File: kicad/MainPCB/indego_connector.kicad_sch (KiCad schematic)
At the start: 20 parts, among them U1 26SHC-B-1A, U2 24SHC-B-1A

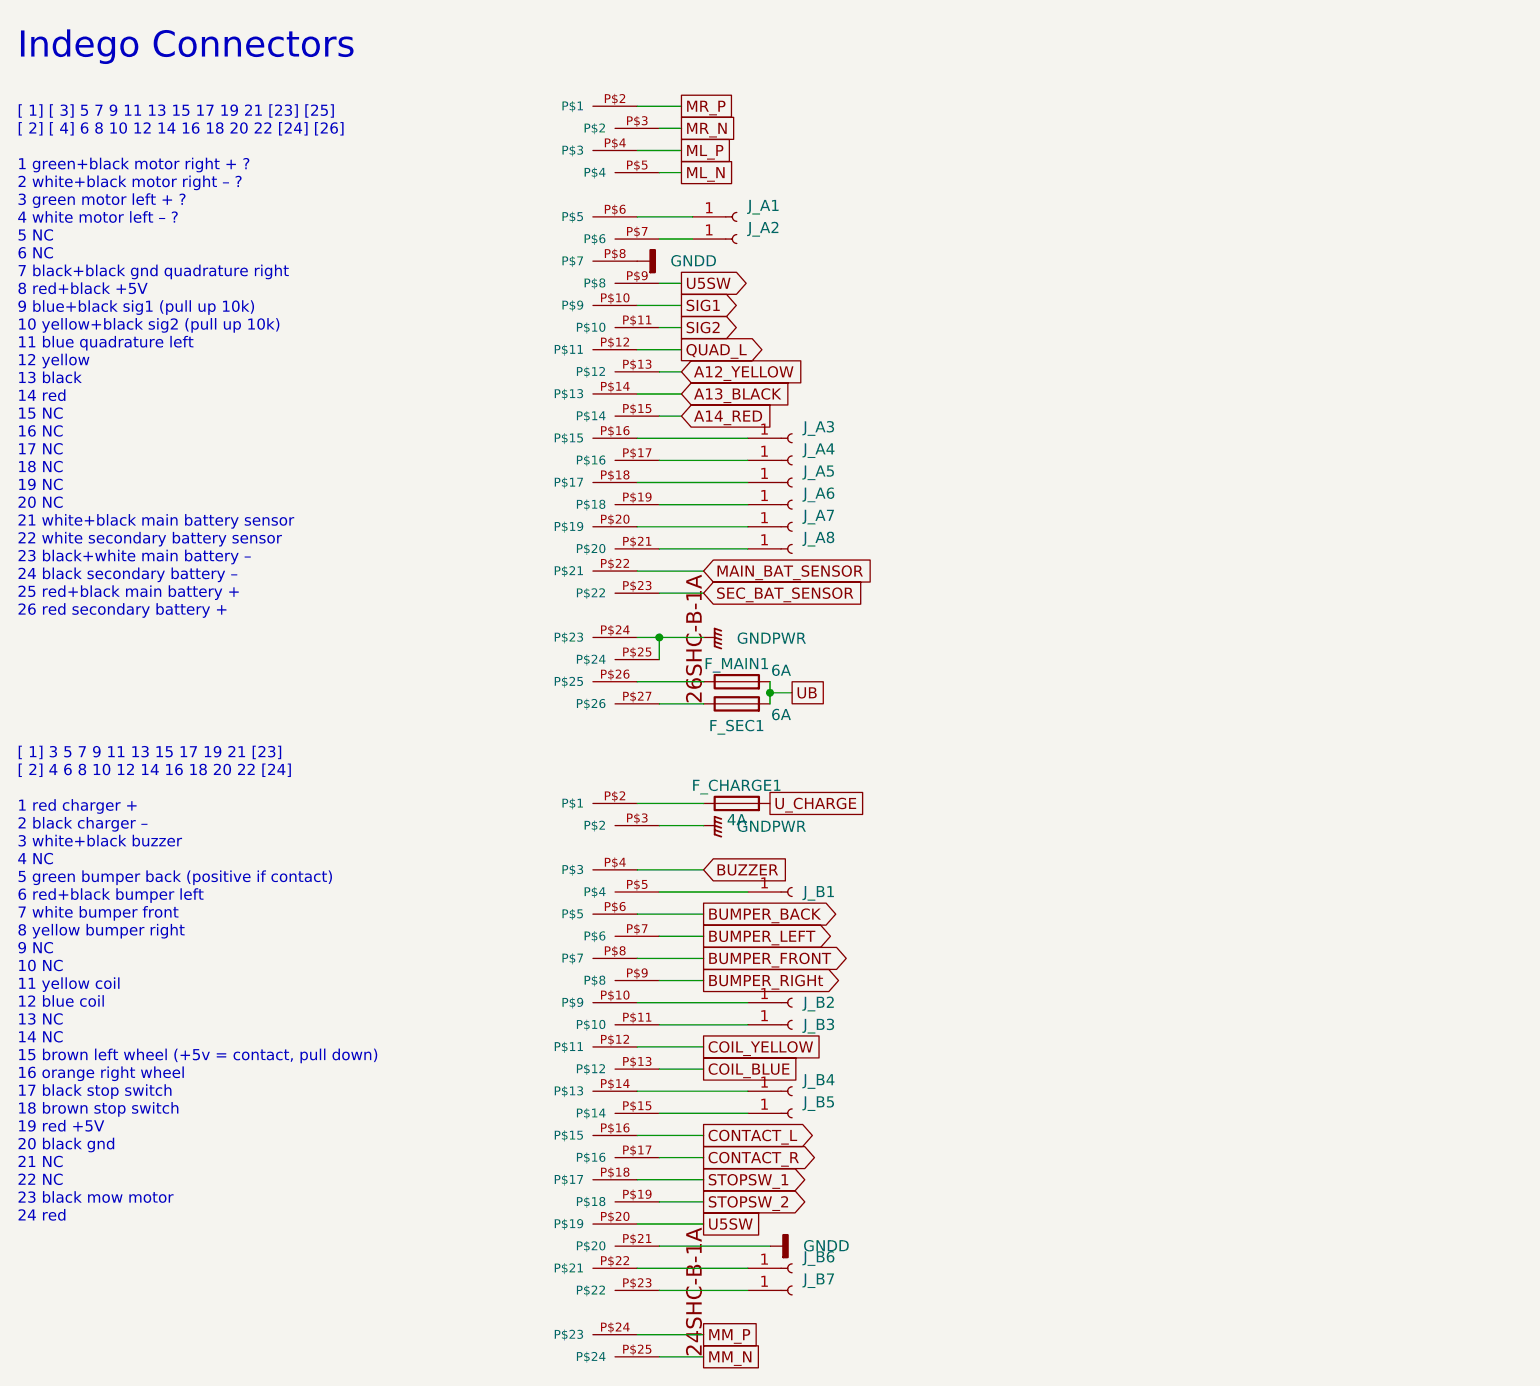
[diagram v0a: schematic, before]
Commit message: some further progress
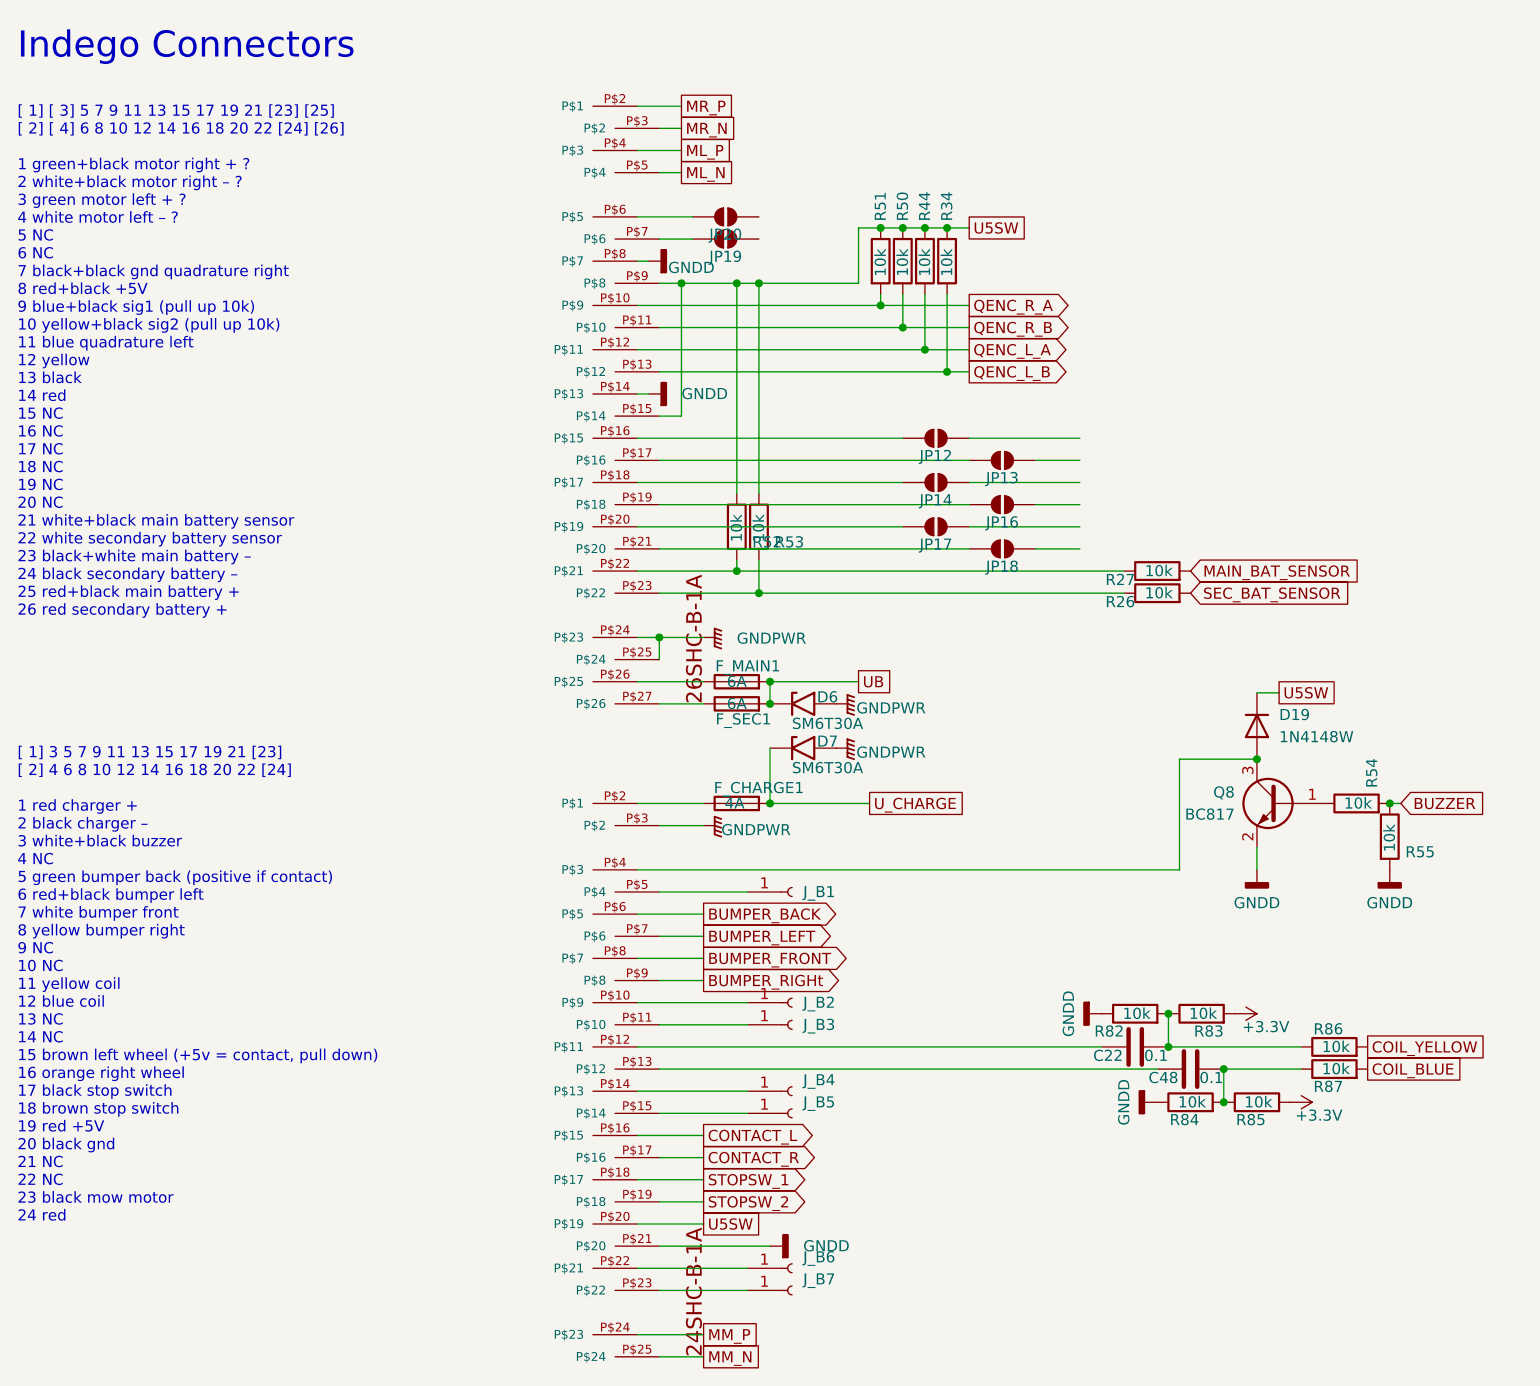
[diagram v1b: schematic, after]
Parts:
- removed J_A1: Conn_01x01_Female, Connector_Wire:SolderWire-0.5sqmm_1x01_D0.9mm_OD2.1mm, symbol Connector:Conn_01x01_Female
- removed J_A2, J_A3, J_A4, J_A5, J_A6, J_A7, J_A8: ~, Connector_Wire:SolderWire-0.5sqmm_1x01_D0.9mm_OD2.1mm, symbol Connector:Conn_01x01_Female
- added C22, C48: 0.1, Capacitor_SMD:C_0805_2012Metric_Pad1.18x1.45mm_HandSolder, symbol Device:C
- added D19: 1N4148W, Diode_SMD:D_SOD-123, symbol Diode:1N4148W
- added D6, D7: SM6T30A, Diode_SMD:D_SMB, symbol Diode:SM6T30A
- added JP12, JP13, JP14, JP16, JP17, JP18, JP19, JP20: SolderJumper_2_Open, symbol Jumper:SolderJumper_2_Open
- added Q8: BC817, Package_TO_SOT_SMD:SOT-23, symbol Transistor_BJT:BC817
- added R26, R27, R34, R44, R50, R51, R52, R53, R54, R55, R82, R83, R84, R85, R86, R87: 10k, Resistor_SMD:R_0805_2012Metric, symbol Device:R
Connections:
- net A13_BLACK is gone; now on net GNDD: U1.P$14 (P$13)
- net A14_RED is gone; now on net U5SW: U1.P$15 (P$14)
- net BUZZER: now also R54.2, R55.1; no longer U2.P$4 (P$3)
- net COIL_BLUE: now also R87.2; no longer U2.P$13 (P$12)
- net COIL_YELLOW: now also R86.2; no longer U2.P$12 (P$11)
- net GNDD: now also Q8.2 (E), R55.2, R82.1, R84.1
- net GNDPWR: now also D6.2 (A2), D7.2 (A2)
- net MAIN_BAT_SENSOR: now also R27.2; no longer U1.P$22 (P$21)
- net SEC_BAT_SENSOR: now also R26.2; no longer U1.P$23 (P$22)
- net U5SW: now also D19.1 (K), R34.1, R44.1, R50.1, R51.1, R52.1, R53.1
- net UB: now also D6.1 (A1)
- net U_CHARGE: now also D7.1 (A1)
- net at U1.P$19 (P$18): now also JP16.1 (A)
- net at U1.P$6 (P$5): now also JP20.1 (A)
- net at U1.P$7 (P$6): now also JP19.1 (A)
- net at U1.P$20 (P$19): now also JP17.1 (A)
- net at U1.P$21 (P$20): now also JP18.1 (A)
- net at U1.P$16 (P$15): now also JP12.1 (A)
- net at U1.P$17 (P$16): now also JP13.1 (A)
- net at U1.P$18 (P$17): now also JP14.1 (A)
- net A12_YELLOW renamed QENC_L_B
- net QENC_L_B: now also R34.2
- net QUAD_L renamed QENC_L_A
- net QENC_L_A: now also R44.2
- net SIG1 renamed QENC_R_A
- net QENC_R_A: now also R51.2
- net SIG2 renamed QENC_R_B
- net QENC_R_B: now also R50.2
- new net: Q8.1 (B), R54.1
- new net: D19.2 (A), Q8.3 (C), U2.P$4 (P$3)
- new net: R26.1, R53.2, U1.P$23 (P$22)
- new net: R27.1, R52.2, U1.P$22 (P$21)
- new net: C22.1, R82.2, R83.1, R86.1
- new net: C22.2, U2.P$12 (P$11)
- new net: C48.1, R84.2, R85.1, R87.1
- new net: C48.2, U2.P$13 (P$12)
- new net +3.3V: R83.2, R85.2
